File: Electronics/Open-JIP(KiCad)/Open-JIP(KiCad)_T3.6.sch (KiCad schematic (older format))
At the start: 31 parts, among them J1 DCJ200-10-A-XX-X_REVA, J2 Screw_Terminal_01x02, U1 74HC4066D,653, U2 74HC4066D,653, U3 KA7812ETU, U4 OPA320AIDBVT, U5 Teensy3.6

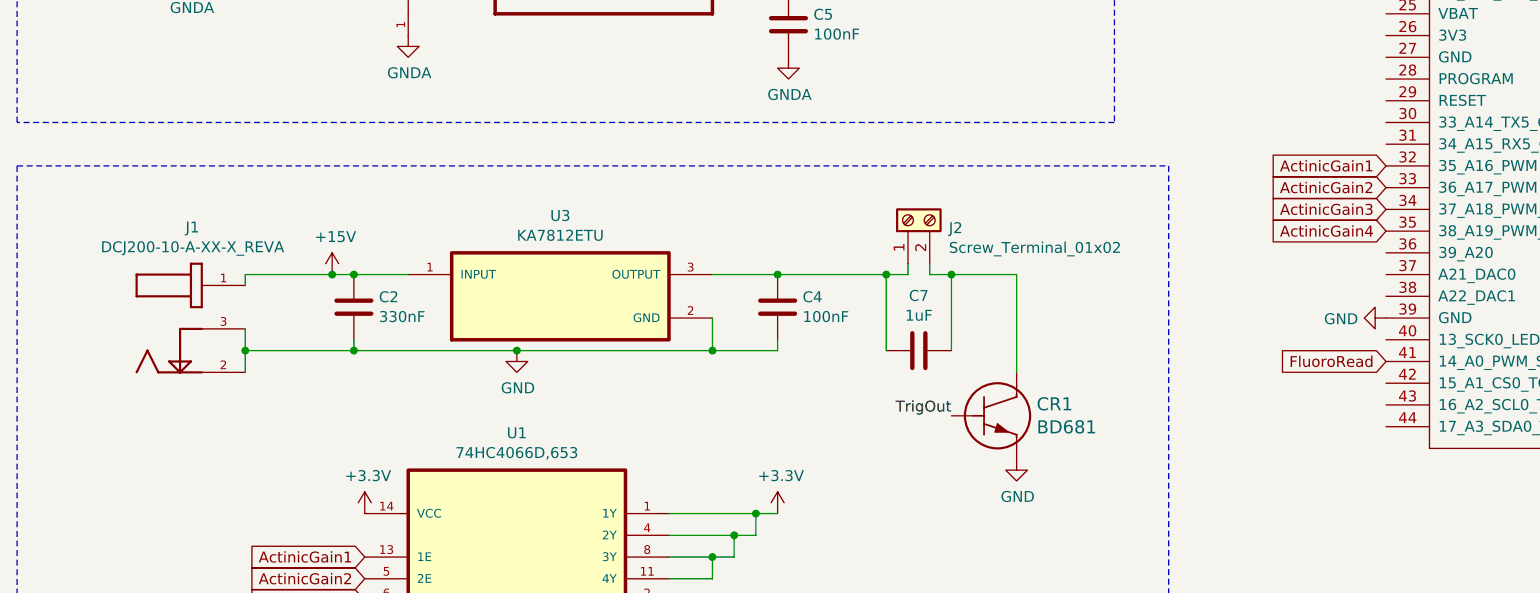
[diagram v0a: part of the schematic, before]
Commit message: finalised v0.3 for teensy 3.6
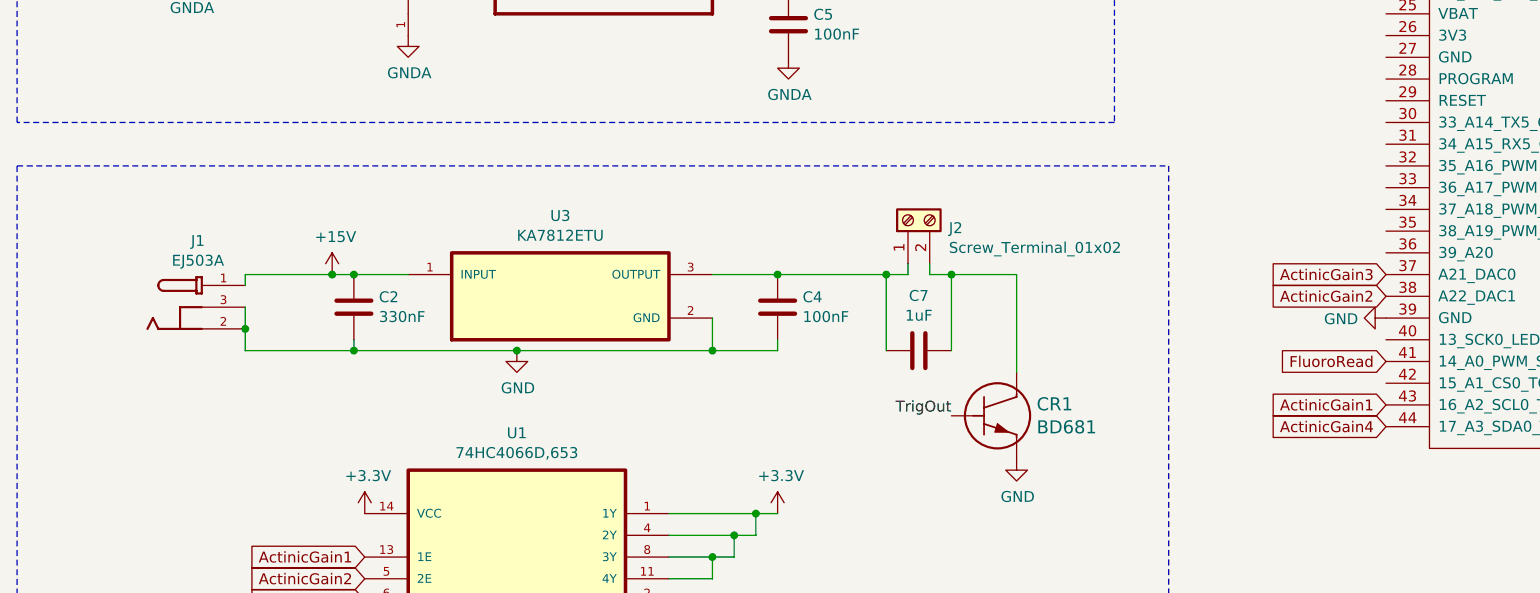
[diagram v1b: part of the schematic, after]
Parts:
- removed J1: DCJ200-10-A-XX-X_REVA, Additional-parts:GCT_DCJ200-10-A-XX-X_REVA, symbol DCJ200-10-A-XX-X_REVA:DCJ200-10-A-XX-X_REVA
- added J1: EJ503A, Additional-parts:DCJack_MPD_EJ503A, symbol DCJack_EJ503A:EJ503A
- U3: footprint TO253P1067X470X2040-3 -> Additional-parts:TO253P1067X470X2040-3
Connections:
- net +15V: now also J1.1
- net ActinicGain1: now also U5.43 (16_A2_SCL0_TOUCH); no longer U5.32 (35_A16_PWM)
- net ActinicGain2: now also U5.38 (A22_DAC1); no longer U5.33 (36_A17_PWM)
- net ActinicGain3: now also U5.37 (A21_DAC0); no longer U5.34 (37_A18_PWM_SCL1)
- net ActinicGain4: now also U5.44 (17_A3_SDA0_TOUCH); no longer U5.35 (38_A19_PWM_SDA1)
- net GND: now also J1.2, J1.3
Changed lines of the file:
@@
-$EndComp
-$Comp
-L DCJ200-10-A-XX-X_REVA:DCJ200-10-A-XX-X_REVA J1
-U 1 1 5FE606E7
-P 1650 5350
-F 0 "J1" H 1707 5817 50  0000 C CNN
-F 1 "DCJ200-10-A-XX-X_REVA" H 1707 5726 50  0000 C CNN
-F 2 "Additional-parts:GCT_DCJ200-10-A-XX-X_REVA" H 1650 5350 50  0001 L BNN
-F 3 "" H 1650 5350 50  0001 L BNN
-F 4 "GCT" H 1650 5350 50  0001 L BNN "MANUFACTURER"
-	1    1650 5350
-	1    0    0    -1
 $EndComp
 $Comp
@@
 F 0 "U3" H 3400 5570 50  0000 C CNN
 F 1 "KA7812ETU" H 3400 5479 50  0000 C CNN
-F 2 "TO253P1067X470X2040-3" H 3400 5200 50  0001 L BNN
+F 2 "Additional-parts:TO253P1067X470X2040-3" H 3400 5200 50  0001 L BNN
 F 3 "" H 3400 5200 50  0001 L BNN
 F 4 "TO253P1067X470X2040-3" H 3400 5200 50  0001 L BNN "Package"
@@
 Wire Wire Line
 	4100 5450 4100 5300
-Connection ~ 1950 5450
-Wire Wire Line
-	1950 5450 1950 5550
 Wire Wire Line
 	2700 5100 2450 5100
@@
 Text GLabel 2500 6700 0    50   Input ~ 0
 ActinicGain4
-Text GLabel 7200 4600 0    50   Input ~ 0
+Text GLabel 7200 5700 0    50   Input ~ 0
 ActinicGain1
-Text GLabel 7200 4700 0    50   Input ~ 0
+Text GLabel 7200 5200 0    50   Input ~ 0
 ActinicGain2
-Text GLabel 7200 4800 0    50   Input ~ 0
+Text GLabel 7200 5100 0    50   Input ~ 0
 ActinicGain3
-Text GLabel 7200 4900 0    50   Input ~ 0
+Text GLabel 7200 5800 0    50   Input ~ 0
 ActinicGain4
 $Comp
@@
 	1    0    0    -1
 $EndComp
+$Comp
+L DCJack_EJ503A:EJ503A J1
+U 1 1 5FE6B45E
+P 1750 5250
+F 0 "J1" H 1732 5555 50  0000 C CNN
+F 1 "EJ503A" H 1732 5464 50  0000 C CNN
+F 2 "Additional-parts:DCJack_MPD_EJ503A" H 1750 5250 50  0001 L BNN
+F 3 "" H 1750 5250 50  0001 L BNN
+F 4 "B" H 1750 5250 50  0001 L BNN "PARTREV"
+F 5 "MPD" H 1750 5250 50  0001 L BNN "MANUFACTURER"
+F 6 "11 mm" H 1750 5250 50  0001 L BNN "MAXIMUM_PACKAGE_HEIGHT"
+F 7 "Manufacturer Recommendations" H 1750 5250 50  0001 L BNN "STANDARD"
+	1    1750 5250
+	1    0    0    -1
+$EndComp
+Wire Wire Line
+	1950 5250 1950 5350
+Connection ~ 1950 5350
 $EndSCHEMATC
